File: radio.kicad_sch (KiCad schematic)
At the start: 60 parts, among them SW3 4*4*1.7, U18 RP2350B, U19 TXM27.12M0004322DBBDO00T, U20 CC1101RGPR, U21 0896BM15A0001001E, U23 EM4095HMSO16B+, U24 PE4259-63, U25 PE4259-63, U26 PE4259-63, U27 PE4259-63, U28 0433BM15A0001001E, U29 PN7160A1HN/C100Y, Y1 12MHz, Y3 26.0MHz

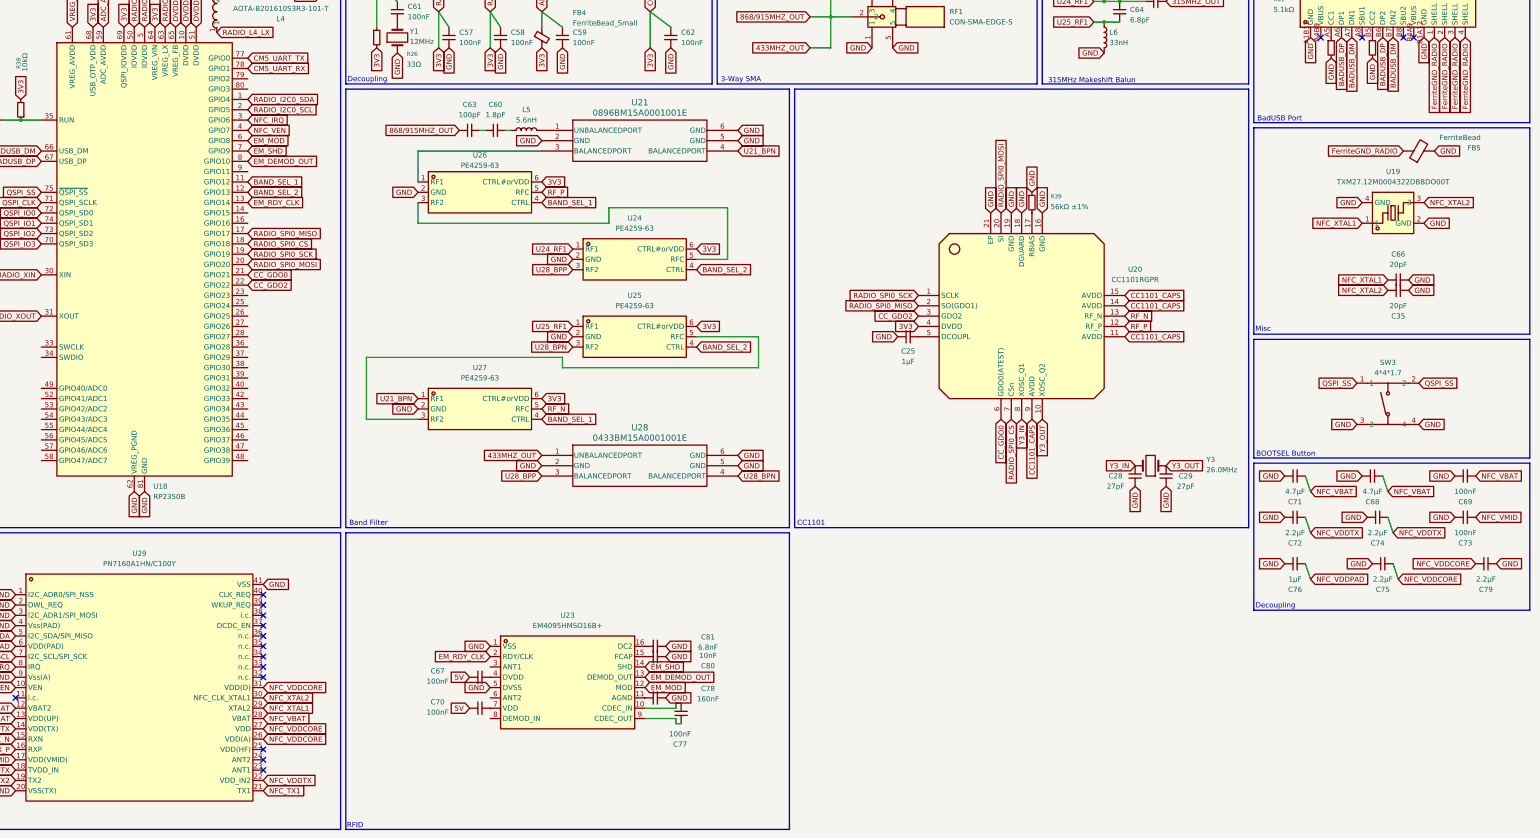
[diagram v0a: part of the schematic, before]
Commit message: finished gps schematic, updated footprints and 3d models
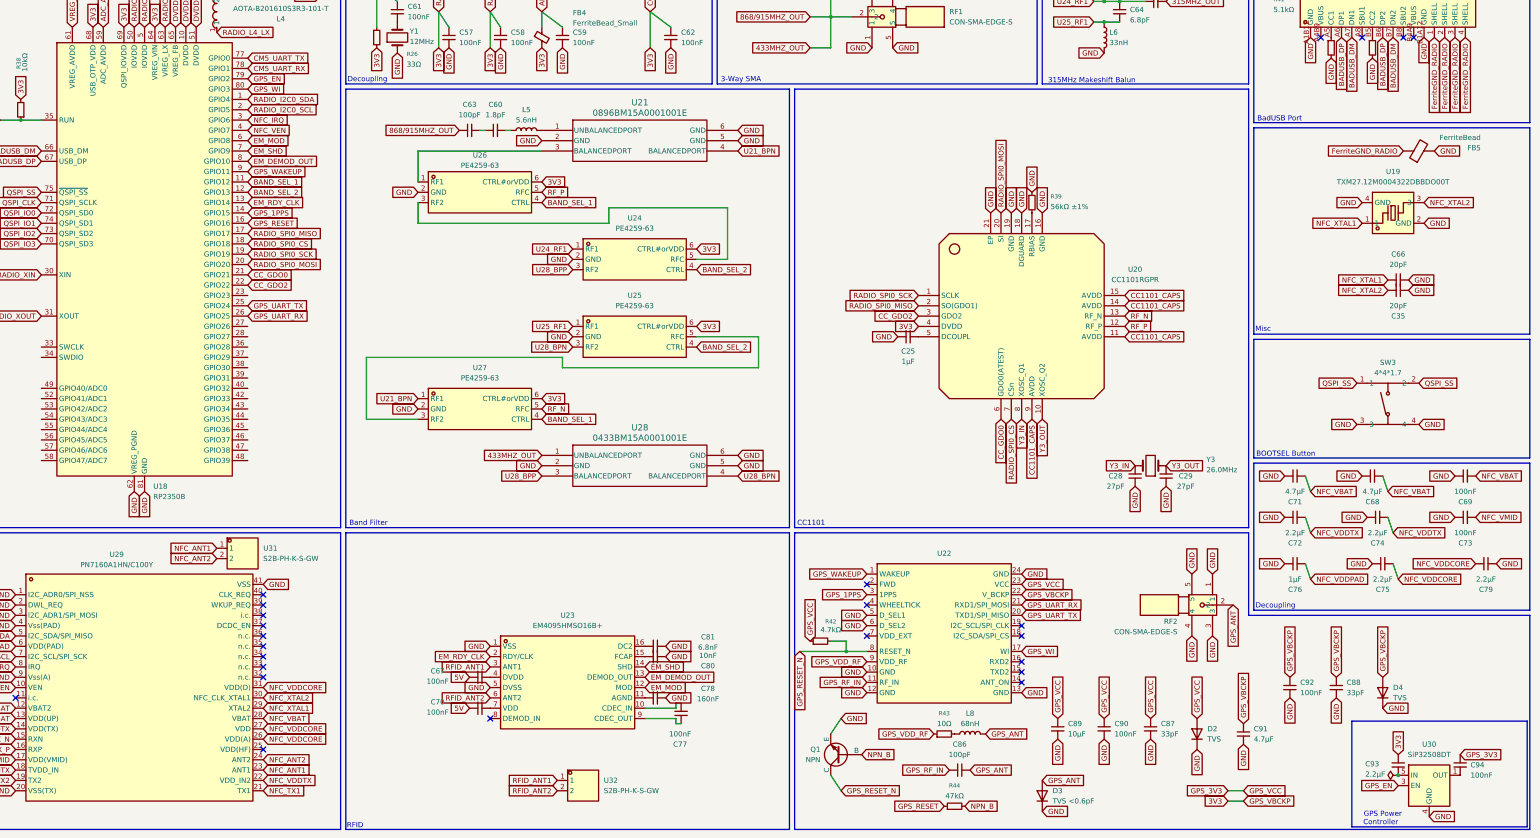
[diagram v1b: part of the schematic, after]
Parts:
- added C86: 100pF, symbol Device:C_Small
- added C87, C88: 33pF, symbol Device:C_Small
- added C89: 10µF, symbol Device:C_Small
- added C90, C92, C94: 100nF, symbol Device:C_Small
- added C91: 4.7µF, symbol Device:C_Small
- added C93: 2.2µF, symbol Device:C_Small
- added D2, D4: TVS, symbol Device:D
- added D3: TVS <0.6pF, symbol Device:D
- added L8: 68nH, symbol Device:L
- added Q1: NPN, symbol Simulation_SPICE:NPN
- added R42: 4.7kΩ, symbol Device:R_Small
- added R43: 10Ω, symbol Device:R_Small
- added R44: 47kΩ, symbol Device:R_Small
- added RF2: CON-SMA-EDGE-S, slate113:SMA-SMD_CON-SMA-EDGE-S, symbol slate113:CON-SMA-EDGE-S
- added U22: (no value), symbol slate113:LC29HCAMD
- added U30: SiP32508DT, Package_TO_SOT_SMD:TSOT-23-6, symbol Power_Management:SiP32508DT
- added U31, U32: S2B-PH-K-S-GW, slate113:CONN-TH_S2B-PH-K-S-GW, symbol slate113:S2B-PH-K-S-GW
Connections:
- net 3V3: now also C88.1, C91.1, C92.1, C93.1, D4.2 (A), U22.22 (V_BCKP)
- net GND: now also C87.2, C88.2, C89.2, C90.2, C91.2, C92.2, D2.1 (K), D3.1 (K), D4.1 (K), Q1.3 (E), RF2.1, RF2.3, RF2.4, RF2.5, U22.10 (GND), U22.12 (GND), U22.13 (GND), U22.24 (GND), U22.5 (D_SEL1), U22.6 (D_SEL2), U30.4 (GND)
- net RFID_ANT1: now reaches U23.3 (ANT1)
- net RFID_ANT1: now also U32.1
- net RFID_ANT2: now reaches U23.6 (ANT2)
- net RFID_ANT2: now also U32.2
- net NFC_ANT1: now reaches U29.23 (ANT1)
- net NFC_ANT1: now also U31.1
- net NFC_ANT2: now reaches U29.24 (ANT2)
- net NFC_ANT2: now also U31.2
- net GPS_1PPS: now reaches U18.14 (GPIO15)
- net GPS_1PPS: now also U22.3 (1PPS)
- net GPS_RESET: now reaches U18.16 (GPIO16)
- net GPS_RESET: now also R44.1
- net GPS_UART_TX: now reaches U18.25 (GPIO24)
- net GPS_UART_TX: now also U22.20 (TXD1/SPI_MISO)
- net GPS_UART_RX: now reaches U18.26 (GPIO25)
- net GPS_UART_RX: now also U22.21 (RXD1/SPI_MOSI)
- net GPS_EN: now reaches U18.79 (GPIO2)
- net GPS_EN: now also U30.3 (EN)
- net GPS_WI: now reaches U18.80 (GPIO3)
- net GPS_WI: now also U22.17 (WI)
- net GPS_WAKEUP: now reaches U18.9 (GPIO11)
- net GPS_WAKEUP: now also U22.1 (WAKEUP)
- new net: L8.1, R43.2
- new net: C94.2, U30.1 (OUT), U30.2 (OUT)
- new net: C93.2, U30.5 (IN), U30.6 (IN)
- new net GPS_3V3: C87.1, C89.1, C90.1, C94.1, D2.2 (A), R42.1, U22.23 (VCC)
- new net GPS_ANT: C86.1, D3.2 (A), L8.2, RF2.2
- new net GPS_RESET_N: Q1.1 (C), R42.2, U22.8 (RESET_N)
- new net GPS_RF_IN: C86.2, U22.11 (RF_IN)
- new net GPS_VDD_RF: R43.1, U22.9 (VDD_RF)
- new net NPN_B: Q1.2 (B), R44.2
- no-connect marks 17 -> 24
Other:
- note added: "Controller"
- note added: "GPS Power"
